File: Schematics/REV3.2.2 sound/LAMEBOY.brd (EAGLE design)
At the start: 45.7 x 67.3 mm, 69 parts, among them IC1 PCF8574T, IC3 MCP73831, Q1 12MHz, U1 USD-SOCKETMICROSDEBAY

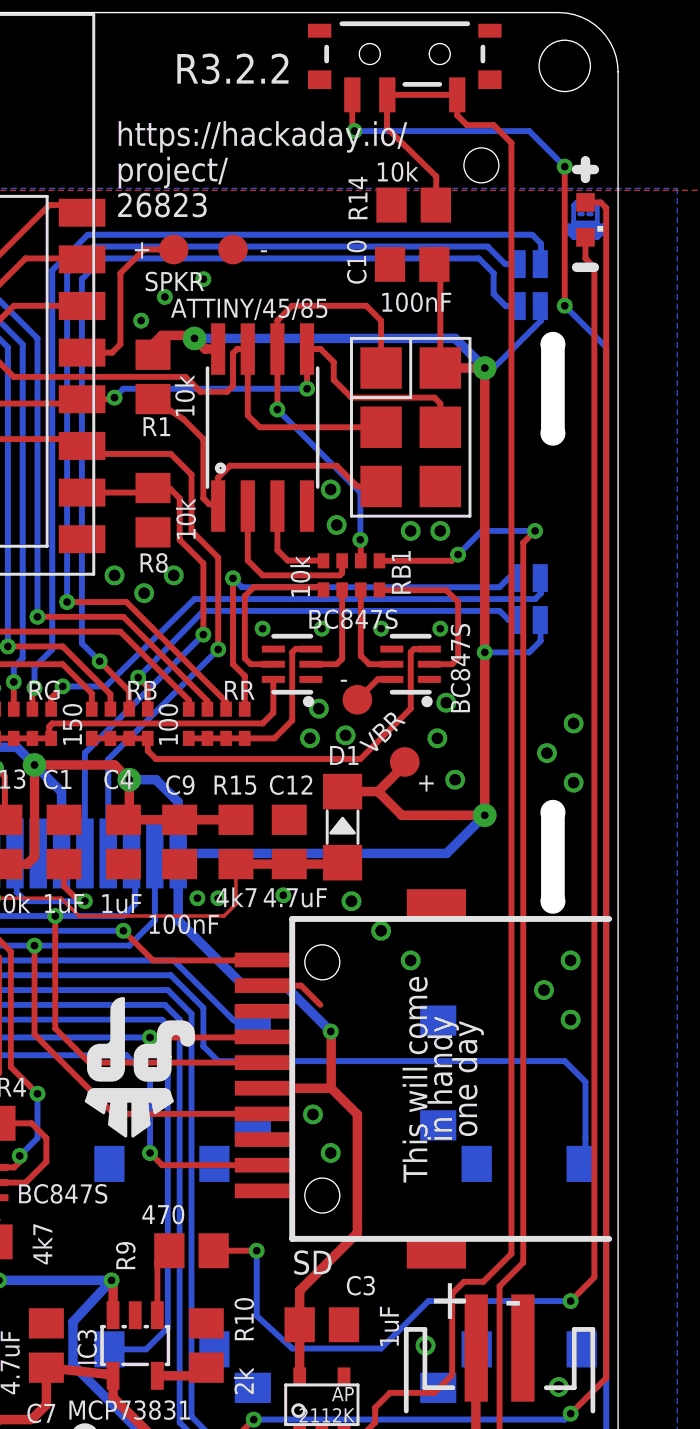
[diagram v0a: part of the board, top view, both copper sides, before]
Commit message: moved labels
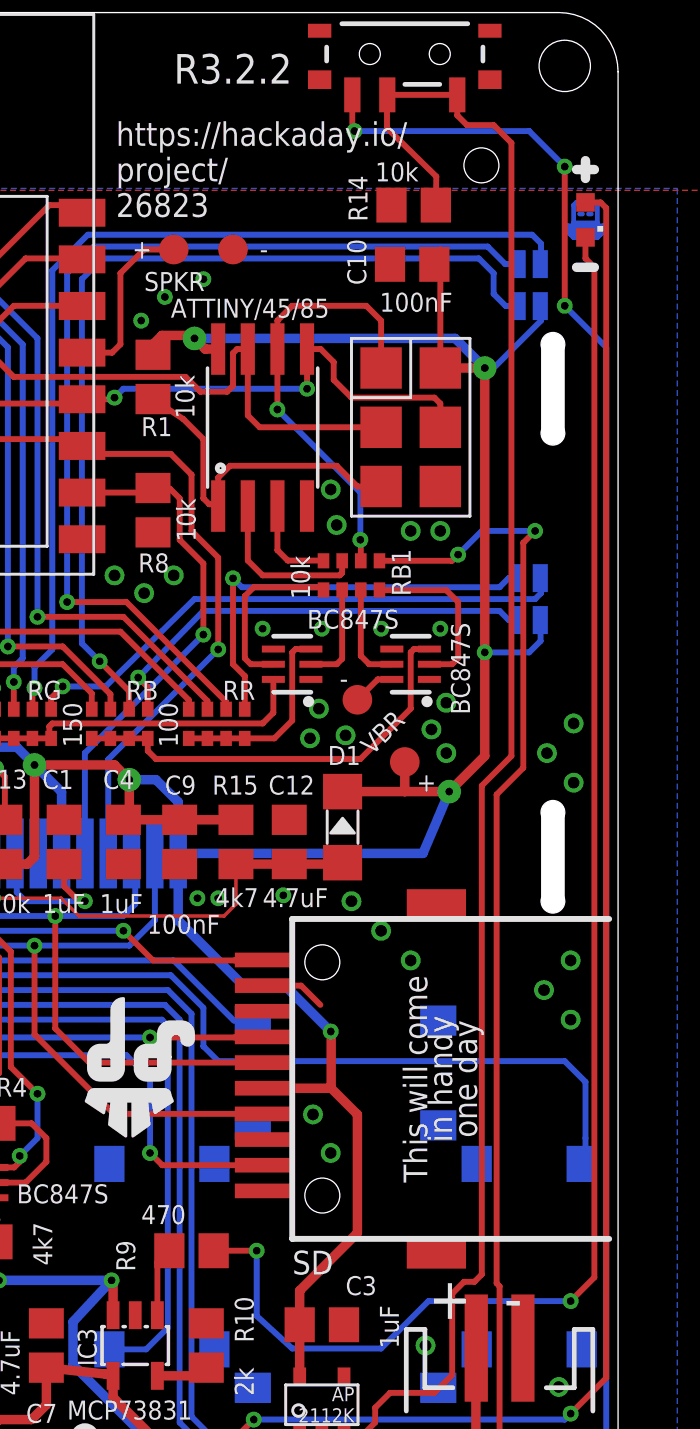
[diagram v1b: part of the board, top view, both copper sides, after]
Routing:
- net VCC: track 235.2 -> 231.9 mm
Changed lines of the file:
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@@
 <via x="42.545" y="25.4" extent="1-16" drill="0.5"/>
 <via x="38.354" y="37.719" extent="1-16" drill="0.5"/>
-<via x="38.735" y="34.417" extent="1-16" drill="0.5"/>
-<via x="37.973" y="36.195" extent="1-16" drill="0.5"/>
+<via x="38.354" y="35.56" extent="1-16" drill="0.5"/>
+<via x="37.719" y="36.576" extent="1-16" drill="0.5"/>
 <via x="34.29" y="29.21" extent="1-16" drill="0.5"/>
 <via x="35.56" y="27.94" extent="1-16" drill="0.5"/>
@@
 <via x="20.701" y="35.052" extent="1-16" drill="0.3302" diameter="1.016"/>
 <wire x1="40.005" y1="52.07" x2="40.005" y2="39.878" width="0.4064" layer="1"/>
-<wire x1="40.005" y1="39.878" x2="40.005" y2="32.893" width="0.4064" layer="1"/>
-<wire x1="26.86091875" y1="31.2592" x2="38.3712" y2="31.2592" width="0.4064" layer="16"/>
-<wire x1="38.3712" y1="31.2592" x2="40.005" y2="32.893" width="0.4064" layer="16"/>
-<via x="40.005" y="32.893" extent="1-16" drill="0.3302" diameter="1.016"/>
+<wire x1="40.005" y1="39.878" x2="40.005" y2="35.433" width="0.4064" layer="1"/>
+<wire x1="40.005" y1="35.433" x2="38.481" y2="33.909" width="0.4064" layer="1"/>
+<wire x1="26.86091875" y1="31.2592" x2="37.3552" y2="31.2592" width="0.4064" layer="16"/>
+<wire x1="37.3552" y1="31.2592" x2="38.481" y2="33.909" width="0.4064" layer="16"/>
+<via x="38.481" y="33.909" extent="1-16" drill="0.3302" diameter="1.016"/>
 <wire x1="21.86091875" y1="31.2592" x2="21.86091875" y2="33.89208125" width="0.4064" layer="16"/>
 <wire x1="21.86091875" y1="33.89208125" x2="20.701" y2="35.052" width="0.4064" layer="16"/>
@@
 <contactref element="D1" pad="C"/>
 <wire x1="26.924" y1="32.7" x2="29.337" y2="32.7" width="0.4064" layer="1"/>
-<wire x1="33.909" y1="33.909" x2="35.433" y2="33.909" width="0.4064" layer="1"/>
-<wire x1="35.433" y1="33.909" x2="36.449" y2="32.893" width="0.4064" layer="1"/>
-<wire x1="36.449" y1="32.893" x2="40.005" y2="32.893" width="0.4064" layer="1"/>
+<wire x1="33.909" y1="33.909" x2="36.576" y2="33.909" width="0.4064" layer="1"/>
+<wire x1="36.576" y1="33.909" x2="38.481" y2="33.909" width="0.4064" layer="1"/>
 <wire x1="32.07" y1="11.049" x2="32.07" y2="12.512" width="0.4064" layer="1"/>
 <wire x1="32.07" y1="12.512" x2="34.544" y2="14.986" width="0.4064" layer="1"/>
@@
 <wire x1="24.13" y1="35.052" x2="20.701" y2="35.052" width="0.4064" layer="1"/>
 <contactref element="TP3" pad="TP"/>
-<wire x1="35.433" y1="33.909" x2="36.322" y2="34.798" width="0.4064" layer="1"/>
-<wire x1="36.322" y1="34.798" x2="36.576" y2="35.179" width="0.4064" layer="1"/>
+<wire x1="36.576" y1="33.909" x2="36.576" y2="35.179" width="0.4064" layer="1"/>
 </signal>
 <signal name="N$8">
@@
 <wire x1="35.826" y1="63.782" x2="38.826" y2="63.782" width="0.254" layer="1"/>
 <wire x1="38.608" y1="12.3825" x2="39.116" y2="12.8905" width="0.254" layer="1"/>
-<wire x1="39.116" y1="12.8905" x2="39.9415" y2="12.8905" width="0.254" layer="1"/>
-<wire x1="39.9415" y1="12.8905" x2="41.148" y2="14.097" width="0.254" layer="1"/>
-<wire x1="41.148" y1="14.097" x2="41.148" y2="61.722" width="0.254" layer="1"/>
+<wire x1="39.116" y1="12.8905" x2="39.5605" y2="12.8905" width="0.254" layer="1"/>
+<wire x1="39.5605" y1="12.8905" x2="39.878" y2="13.208" width="0.254" layer="1"/>
+<wire x1="39.878" y1="13.208" x2="39.878" y2="34.163" width="0.254" layer="1"/>
+<wire x1="39.878" y1="34.163" x2="41.148" y2="35.433" width="0.254" layer="1"/>
+<wire x1="41.148" y1="35.433" x2="41.148" y2="61.722" width="0.254" layer="1"/>
 <wire x1="41.148" y1="61.722" x2="40.386" y2="62.484" width="0.254" layer="1"/>
 <wire x1="33.97" y1="6.42" x2="34.868" y2="6.42" width="0.254" layer="1"/>
@@
 <contactref element="IC1" pad="4"/>
 <via x="40.64" y="2.286" extent="1-16" drill="0.3302"/>
-<wire x1="41.656" y1="44.577" x2="41.656" y2="13.716" width="0.254" layer="1"/>
+<wire x1="41.656" y1="44.577" x2="41.656" y2="34.925" width="0.254" layer="1"/>
+<wire x1="41.656" y1="34.925" x2="40.513" y2="33.782" width="0.254" layer="1"/>
+<wire x1="40.513" y1="33.782" x2="40.513" y2="12.827" width="0.254" layer="1"/>
 <wire x1="40.64" y1="2.286" x2="37.084" y2="2.286" width="0.254" layer="16"/>
 <wire x1="37.084" y1="2.286" x2="36.576" y2="2.794" width="0.254" layer="16"/>
@@
 <wire x1="28.067" y1="5.715" x2="26.924" y2="6.858" width="0.254" layer="16"/>
 <wire x1="40.64" y1="2.286" x2="40.64" y2="12.7" width="0.254" layer="1"/>
-<wire x1="40.64" y1="12.7" x2="41.656" y2="13.716" width="0.254" layer="1"/>
+<wire x1="40.64" y1="12.7" x2="40.513" y2="12.827" width="0.254" layer="1"/>
 <contactref element="RB1" pad="5"/>
 <wire x1="35.49" y1="43.805" x2="38.598" y2="43.805" width="0.254" layer="1"/>
